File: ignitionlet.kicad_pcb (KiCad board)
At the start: 4 copper layers, 153.7 x 43.2 mm, 145 parts, among them J1 Conn_Coaxial, J10 Conn_Coaxial, J101 Barrel_Jack_MountingPin, J102 Conn_01x02, J103 Conn_01x03, J11 Conn_Coaxial, J12 Conn_Coaxial, J13 Conn_02x06_Odd_Even, J14 Conn_02x06_Odd_Even, J15 Conn_01x04, J16 Conn_02x06_Top_Bottom, J17 Conn_01x04, J2 Conn_Coaxial, J201 PMOD_2A_PERIPHERAL, J202 IGNITION_TARGET_HDR, J203 Conn_02x04_Odd_Even, J204 Conn_01x03, J205 Conn_01x03, J3 Conn_Coaxial, J4 Conn_Coaxial, J5 Conn_01x04, J6 Conn_01x04, J7 Conn_01x04, J8 Conn_01x04, J9 Conn_Coaxial, SW1 FPGA_RST, SW2 SYS_RST, SW3 FLT, U1 IGNITION001-QFN, U101 LT3013EFE#PBF, U102 LT3013EFE#PBF, U103 TPS7A0525PDBVR, U2 AMPMGFB-50.0000T, U5 MT25QL128ABB8E12-0AUT, U6 AT25PE80-SSHN-B

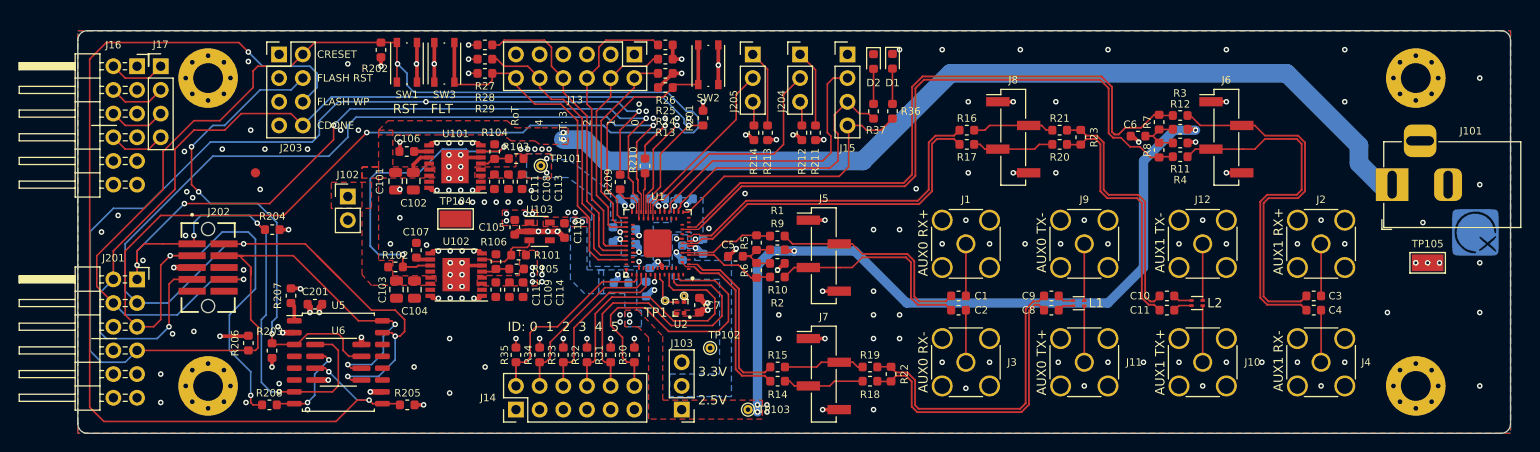
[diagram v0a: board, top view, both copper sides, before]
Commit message: Ignitionlet rev 2, first pass
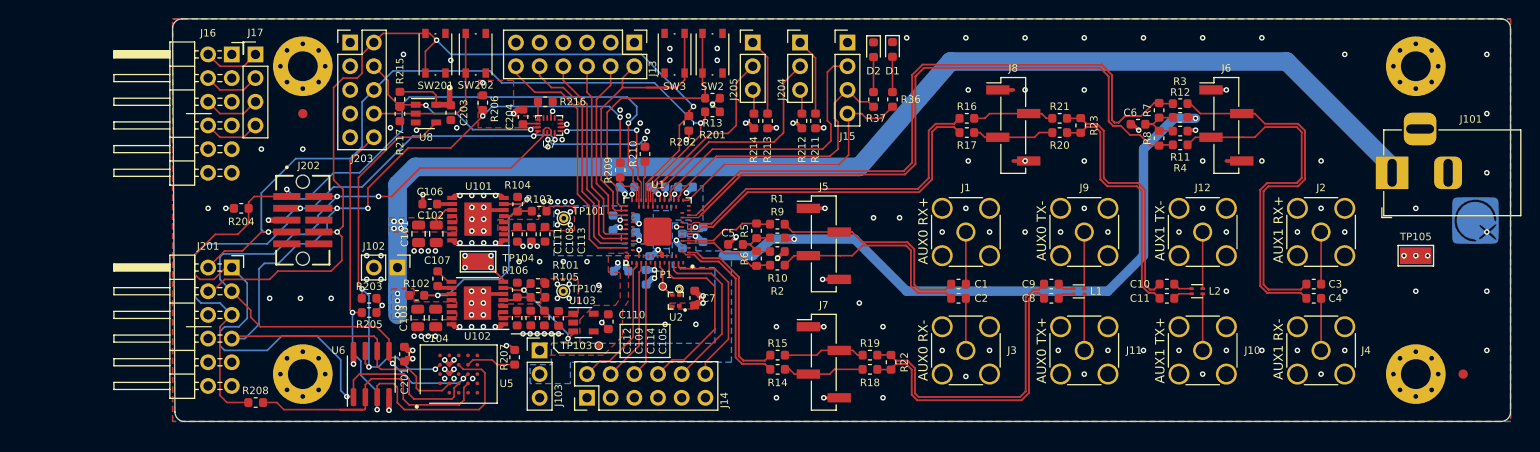
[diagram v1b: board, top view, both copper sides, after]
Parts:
- removed R24, R25, R26, R27, R28, R29, R30, R31, R32, R33, R34, R35: 10K, Resistor_SMD:R_0603_1608Metric
- removed SW1: FPGA_RST, c-and-k-pts851:PTS815
- added C203: GCM188R71E105KA64D, Capacitor_SMD:C_0603_1608Metric, F.Cu at (104.8, 81.2)
- added C204: GCM188R71E105KA64D, Capacitor_SMD:C_0603_1608Metric, F.Cu at (112.5, 81.6)
- added FID3: Fiducial, Fiducial:Fiducial_1mm_Mask2mm, F.Cu at (213.4, 109.2)
- added R215: 10K, Resistor_SMD:R_0603_1608Metric, F.Cu at (99.3, 79.7)
- added R216: 10K, Resistor_SMD:R_0603_1608Metric, F.Cu at (114.9, 80.0)
- added R217: 10K, Resistor_SMD:R_0603_1608Metric, F.Cu at (99.3, 81.3)
- added SW201: FPGA_RST, c-and-k-pts851:PTS815, F.Cu at (103.1, 74.9)
- added SW202: FLASH_RST, c-and-k-pts851:PTS815, F.Cu at (107.4, 74.9)
- added U7: SN74CBTLV3257RSV, Package_DFN_QFN_0x:Texas_RSV_S-UQFN-16_2.4x1.6mm, F.Cu at (115.3, 82.5)
- added U8: SN74AUP1G08DBVR, Package_TO_SOT_SMD:SOT-23-5, F.Cu at (102.1, 81.3)
- FID1: footprint grumpy:Oxide_Board_Identifier_23x6mm -> grumpy:Oxide_Board_Identifier_23x6mm_PCBWay
- J203: value Conn_02x04_Odd_Even -> Conn_02x05_Odd_Even; footprint Connector_PinHeader_2.54mm:PinHeader_2x04_P2.54mm_Vertical -> Connector_PinHeader_2.54mm:PinHeader_2x05_P2.54mm_Vertical
- R36, R37: value 280 -> 309
- TP1: footprint test-point:TestPoint_THTPad_D0.6mm_Drill0.3mm -> test-point:TestPoint_Pad_D0.6mm
- TP103: footprint TestPoint:TestPoint_THTPad_D1.0mm_Drill0.5mm -> test-point:TestPoint_Pad_D0.6mm
- U5: footprint micron-sop2:Micron_SOP2-16_7.5x10.3mm_P1.27mm -> Package_BGA_0x:T-PBGA-24_6x8mm_Layout5x5_P1.0mm
- moved R206 36.0 mm to (108.2, 80.1)
- moved R202 33.9 mm to (130.3, 82.3)
- moved R207 24.9 mm to (111.6, 107.4)
- moved SW3 24.7 mm to (128.8, 74.9)
- moved TP103 17.4 mm to (120.7, 106.2)
- moved TP102 16.9 mm to (116.8, 100.3)
- moved J103 16.5 mm to (114.3, 106.7), turned to 0 degrees
- moved U5 13.0 mm to (105.6, 109.2), turned to 90 degrees
- moved R203 11.8 mm to (96.0, 101.1), turned to 0 degrees
- moved J202 11.4 mm to (88.9, 92.7)
- moved C201 11.0 mm to (99.8, 107.1), turned to 90 degrees
- moved C105 10.8 mm to (116.3, 103.3)
- moved C110 10.8 mm to (121.7, 103.6)
- moved U103 10.8 mm to (119.0, 103.7)
- moved R205 10.7 mm to (96.0, 102.6)
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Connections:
- net /Config/~FPGA_RESET renamed /Config/SPI_RESET_L
- C120 pad 1: /Power/VCCIO_3 -> VCCIO_3
- J103 pad 2: /Power/VCCIO_3 -> VCCIO_3
- J201 pad 1: /Config/~SPI_SS -> /Config/SPI_SS_L
- J201 pad 7: /Config/CDONE -> /Config/FPGA_CDONE
- J202 pad 1: /Config/~SPI_SS -> /Config/SPI_SS_L
- J202 pad 7: /Config/CDONE -> /Config/FPGA_CDONE
- J203 pad 4: /Config/~FLASH_RESET -> /Config/FPGA_MODE
- J203 pad 5: GND -> Net-(J203-Pad5)
- J203 pad 6: /Config/~FLASH_WP -> /Config/FPGA_CDONE
- J203 pad 7: Net-(J203-Pad7) -> GND
- J203 pad 8: /Config/CDONE -> /Config/FLASH_RESET_JP_L
- R11 pad 1: V2P5 -> VCCIO_3
- R201 pad 1: /Config/CDONE -> /Config/FPGA_CDONE
- R203 pad 1: /Config/~FLASH_RESET -> /Config/FLASH_RESET_L
- R204 pad 1: /Config/~SPI_SS -> /Config/SPI_SS_L
- R205 pad 1: /Config/~FLASH_WP -> /Config/FLASH_WP_L
- R207 pad 1: /Config/~FLASH_HOLD -> /Config/FLASH_HOLD_L
- R208 pad 1: /Config/FLASH_DO -> /Config/FLASH_MISO
- R210 pad 2: /Config/SPI_MISO -> /Config/FPGA_MOSI
- R9 pad 1: V2P5 -> VCCIO_3
- SW3 pad 1: /~ROT_FLT -> /~PWR_FLT0
- U1 pad A22: /Config/SPI_MOSI -> /Config/FPGA_MISO
- U1 pad B16: /Config/CDONE -> /Config/FPGA_CDONE
- U1 pad B18: /Config/~SPI_SS -> /Config/SPI_SS_L
- U1 pad B6: /Power/VCCIO_3 -> VCCIO_3
- U6 pad 1: /Config/~SPI_SS -> /Config/SPI_SS_L
- U6 pad 2: /Config/FLASH_DO -> /Config/FLASH_MISO
- U6 pad 3: /Config/~FLASH_WP -> /Config/FLASH_WP_L
- U6 pad 7: /Config/~FLASH_RESET -> /Config/FLASH_RESET_L
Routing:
- net /Config/~SPI_SS: track 130.2 -> 0.00 mm, vias 7 -> 0
- net /Config/SPI_SS_L: track 0.00 -> 125.1 mm, vias 0 -> 3
- net /Config/CDONE: track 111.8 -> 0.00 mm, vias 2 -> 0
- net /Config/~FLASH_WP: track 109.8 -> 0.00 mm, vias 3 -> 0
- net /Config/FPGA_CDONE: track 0.00 -> 85.2 mm, vias 0 -> 2
- net V2P5: track 82.6 -> 1.61 mm, vias 9 -> 1
- net VCCIO_3: track 0.00 -> 70.6 mm, vias 0 -> 3
- net /Config/SPI_SCK: track 154.5 -> 94.0 mm
- net /Config/FLASH_WP_L: track 0.00 -> 55.5 mm, vias 0 -> 2
- net /Config/~FLASH_RESET: track 54.9 -> 0.00 mm, vias 3 -> 0
- net /Config/SPI_MISO: track 124.0 -> 69.3 mm, vias 4 -> 3
- net /Config/SPI_MOSI: track 134.9 -> 80.3 mm
- net /Config/FLASH_RESET_L: track 0.00 -> 43.2 mm, vias 0 -> 3
- net /Config/FLASH_MISO: track 0.00 -> 31.5 mm
- net VIN_12V: track 103.4 -> 134.5 mm, vias 2 -> 8
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- added copper zone on B.Cu, net VCCIO_3
- removed copper zone on B.Cu, net /Power/VCCIO_3
- removed copper zone on B.Cu, net V2P5
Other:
- board size 153.7 x 43.2 mm -> 143.5 x 43.2 mm
- board text removed: "2.5V"
- board text removed: "3.3V"
- board text removed: "CDONE"
- board text removed: "CRESET"
- board text removed: "FLASH RST"
- board text removed: "FLASH WP"
- board text removed: "FLT"
- board text removed: "ID: 0 1 2 3 4 5"
- board text removed: "RST"
- board text removed: "RoT 4 FLT: 3 2 1 0"
